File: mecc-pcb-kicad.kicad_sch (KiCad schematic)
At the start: 54 parts, among them J1 VESC Term, J2 VBatt -> 5V, J3 Wave_Gauge, J4 5V -> 3.3V, J5 PDQE15-Q48-D24-D, J6 VESC IN, J7 UI BUS, J8 Torq_SENS, Q1 NMOS, Q2 NMOS, Q3 PMOS, Q4 PMOS, SW1 Reset, U1 SEN-16407, U2 SN74HCS09QPWRQ1, U3 SN74LVC1G139DCUR

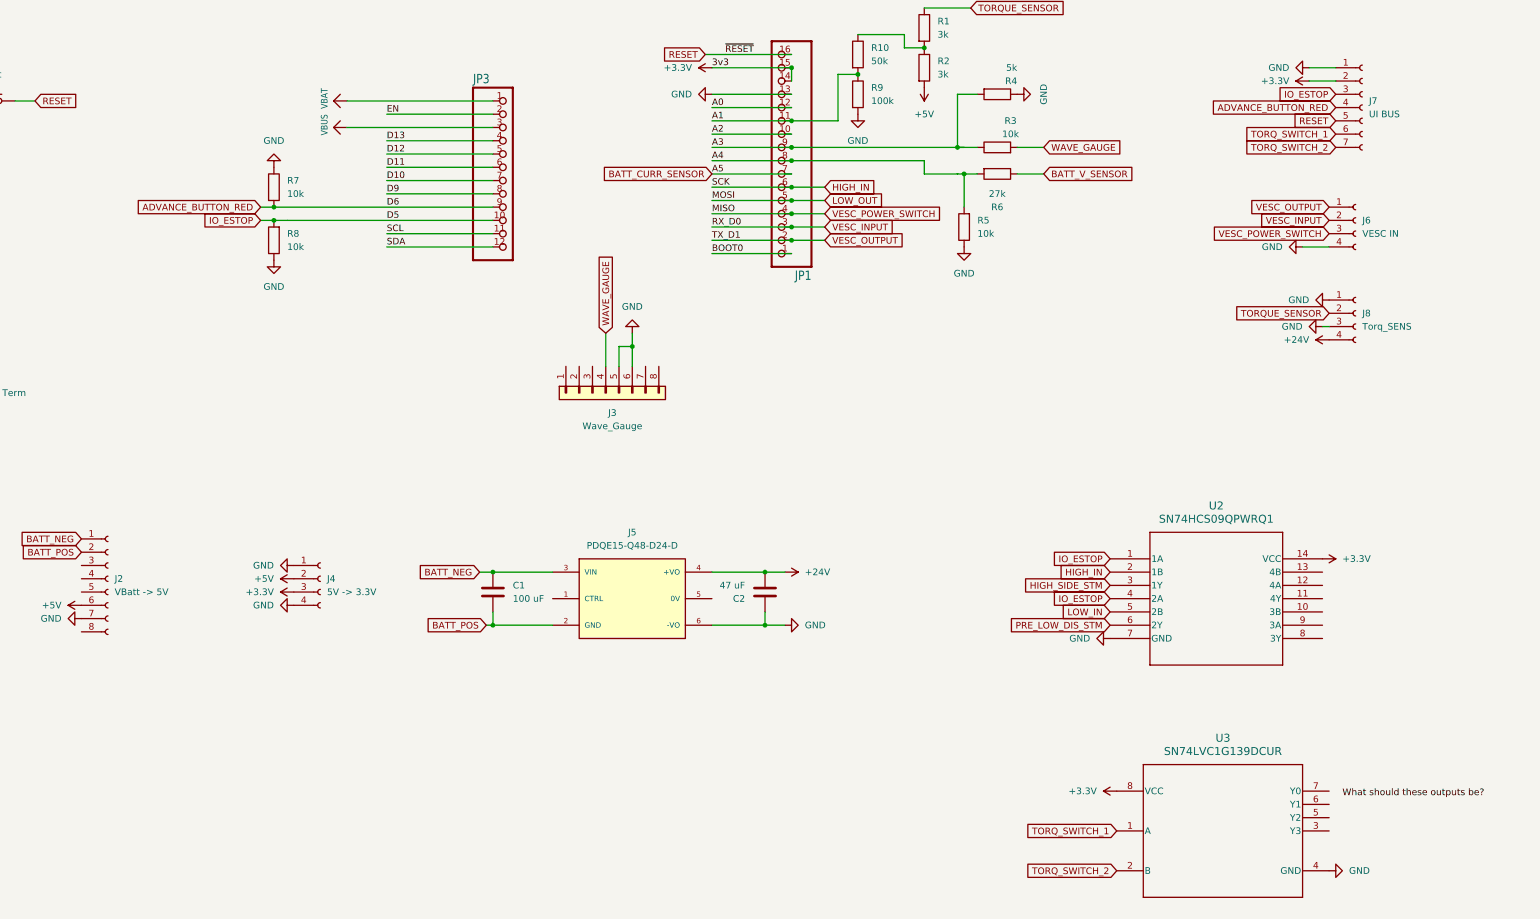
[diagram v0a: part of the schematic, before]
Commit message: Implemented some of becca's changes
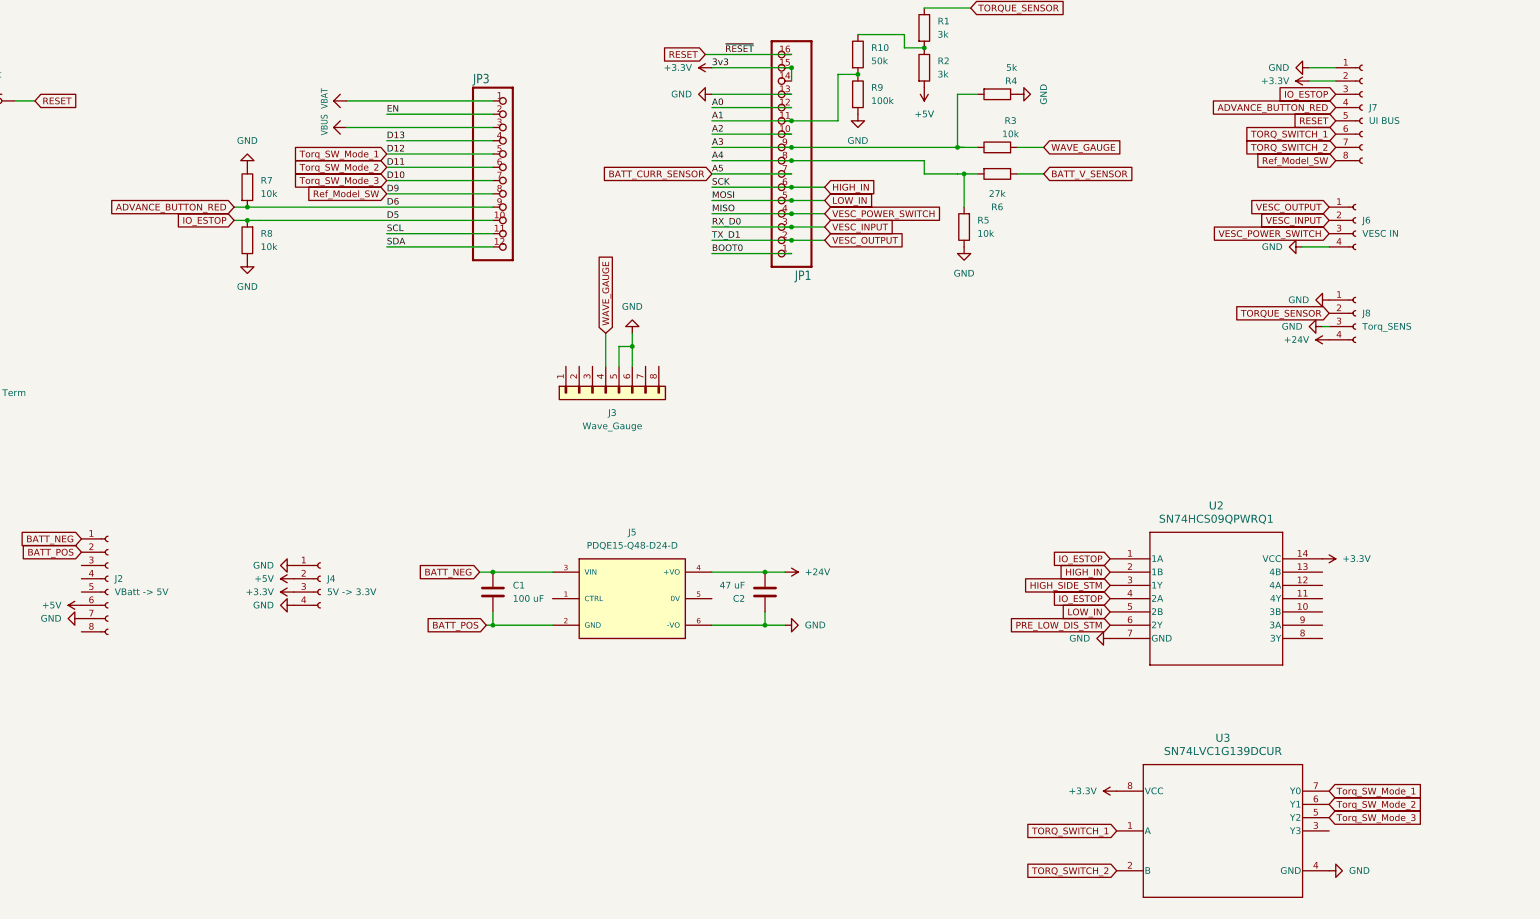
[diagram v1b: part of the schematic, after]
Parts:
- J7: footprint Connector_Molex:Molex_KK-254_AE-6410-07A_1x07_P2.54mm_Vertical -> Connector_Molex:Molex_KK-254_AE-6410-08A_1x08_P2.54mm_Vertical; symbol Connector:Conn_01x07_Socket -> Connector:Conn_01x08_Socket
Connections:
- net D10 is gone; now on net Torq_SW_Mode_3: JP3.7
- net D11 is gone; now on net Torq_SW_Mode_2: JP3.6
- net D12 is gone; now on net Torq_SW_Mode_1: JP3.5
- net LOW_OUT is gone; now on net LOW_IN: JP1.5
- net Torq_SW_Mode_3: now reaches U3.5 (Y2)
- net Torq_SW_Mode_2: now reaches U3.6 (Y1)
- net Torq_SW_Mode_1: now reaches U3.7 (Y0)
- net D9 renamed Ref_Model_SW
- net Ref_Model_SW: now also J7.8 (Pin_8)
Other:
- moved on the sheet: R7, R8

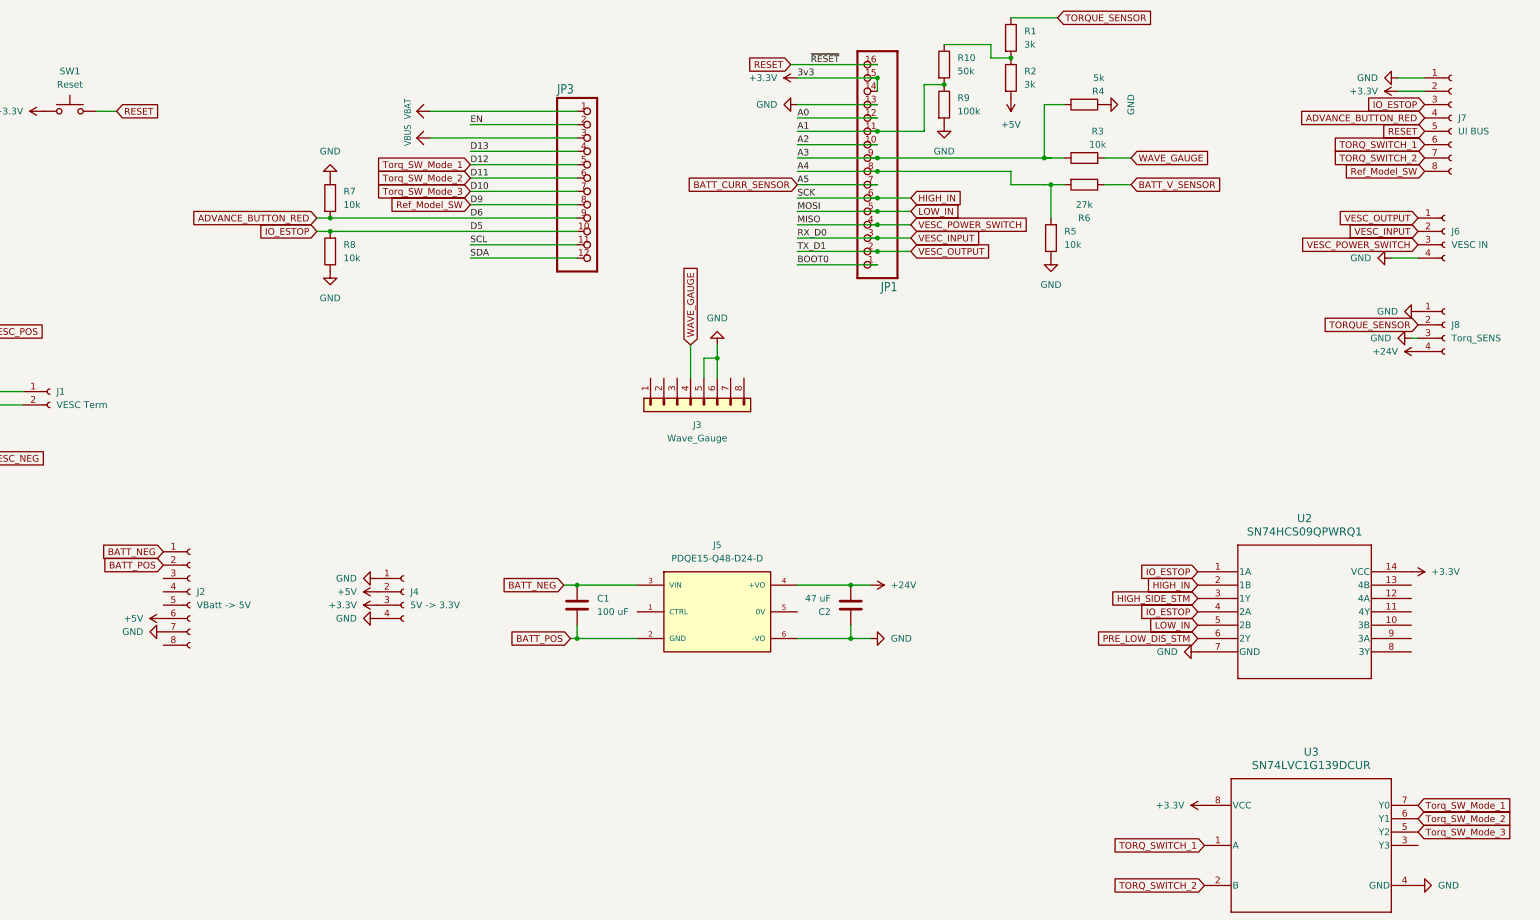
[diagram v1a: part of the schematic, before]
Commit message: I don't even think I made changes I'm just paranoid
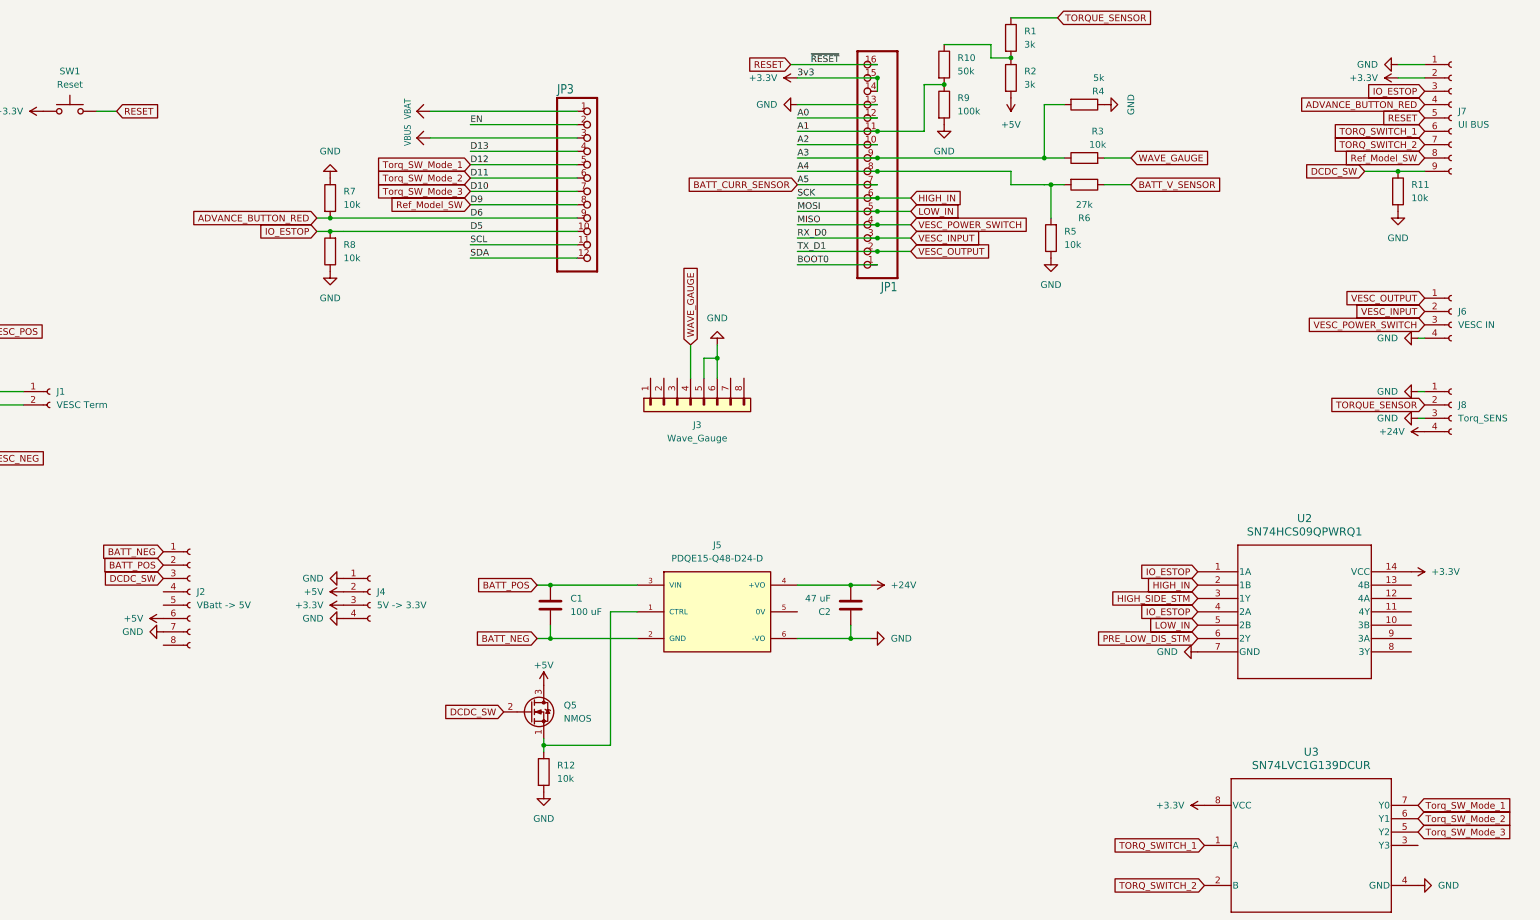
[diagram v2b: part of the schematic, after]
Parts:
- added Q5: NMOS, Library:WEC_NMOS, symbol Transistor_FET:2N7000
- added R11, R12: 10k, Resistor_THT:R_Axial_DIN0204_L3.6mm_D1.6mm_P7.62mm_Horizontal, symbol Device:R
- J7: symbol Connector:Conn_01x08_Socket -> Connector:Conn_01x09_Socket
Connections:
- net +5V: now also Q5.3 (D)
- net BATT_NEG: now also C1.2, J5.2 (GND); no longer C1.1, J5.3 (VIN)
- net BATT_POS: now also C1.1, J5.3 (VIN); no longer C1.2, J5.2 (GND)
- net GND: now also R11.2, R12.2
- net DCDC_SW: now reaches J2.3 (Pin_3)
- net DCDC_SW: now also J7.9 (Pin_9), Q5.2 (G), R11.1
- net at J5.1 (CTRL): now also Q5.1 (S), R12.1
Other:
- moved on the sheet: C1, J4, J6, J8
